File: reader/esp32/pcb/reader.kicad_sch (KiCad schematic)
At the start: 12 parts, among them U1 ESP32-WROOM-32U, U2 RDM6300

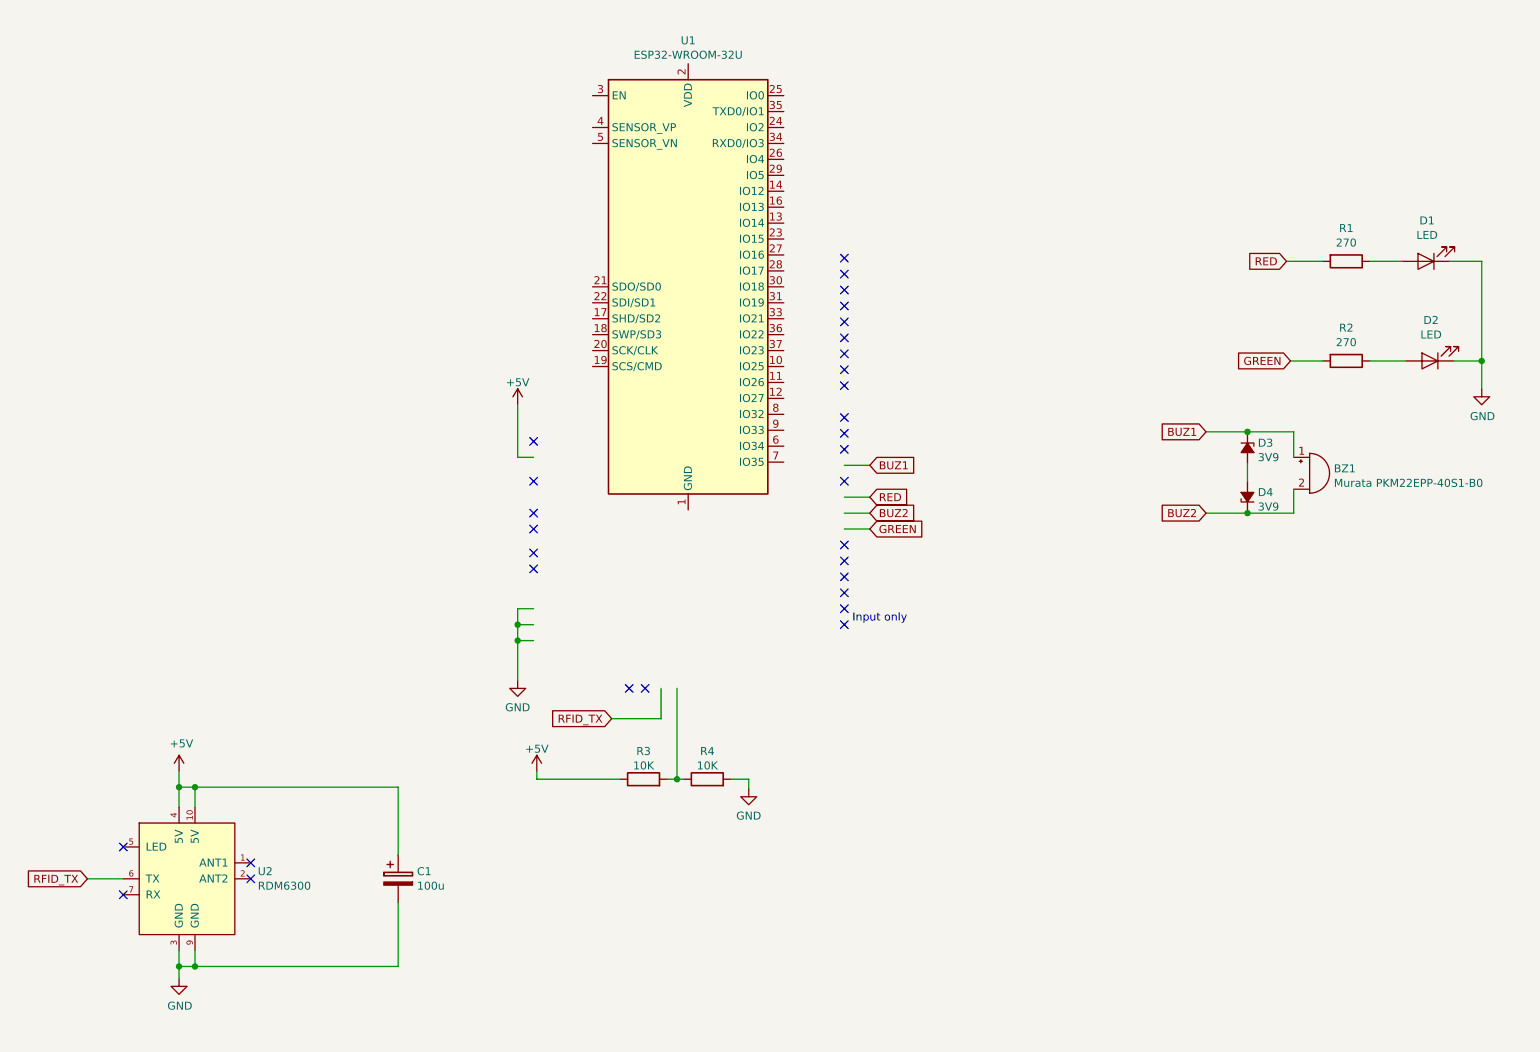
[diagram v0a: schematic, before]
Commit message: Work.
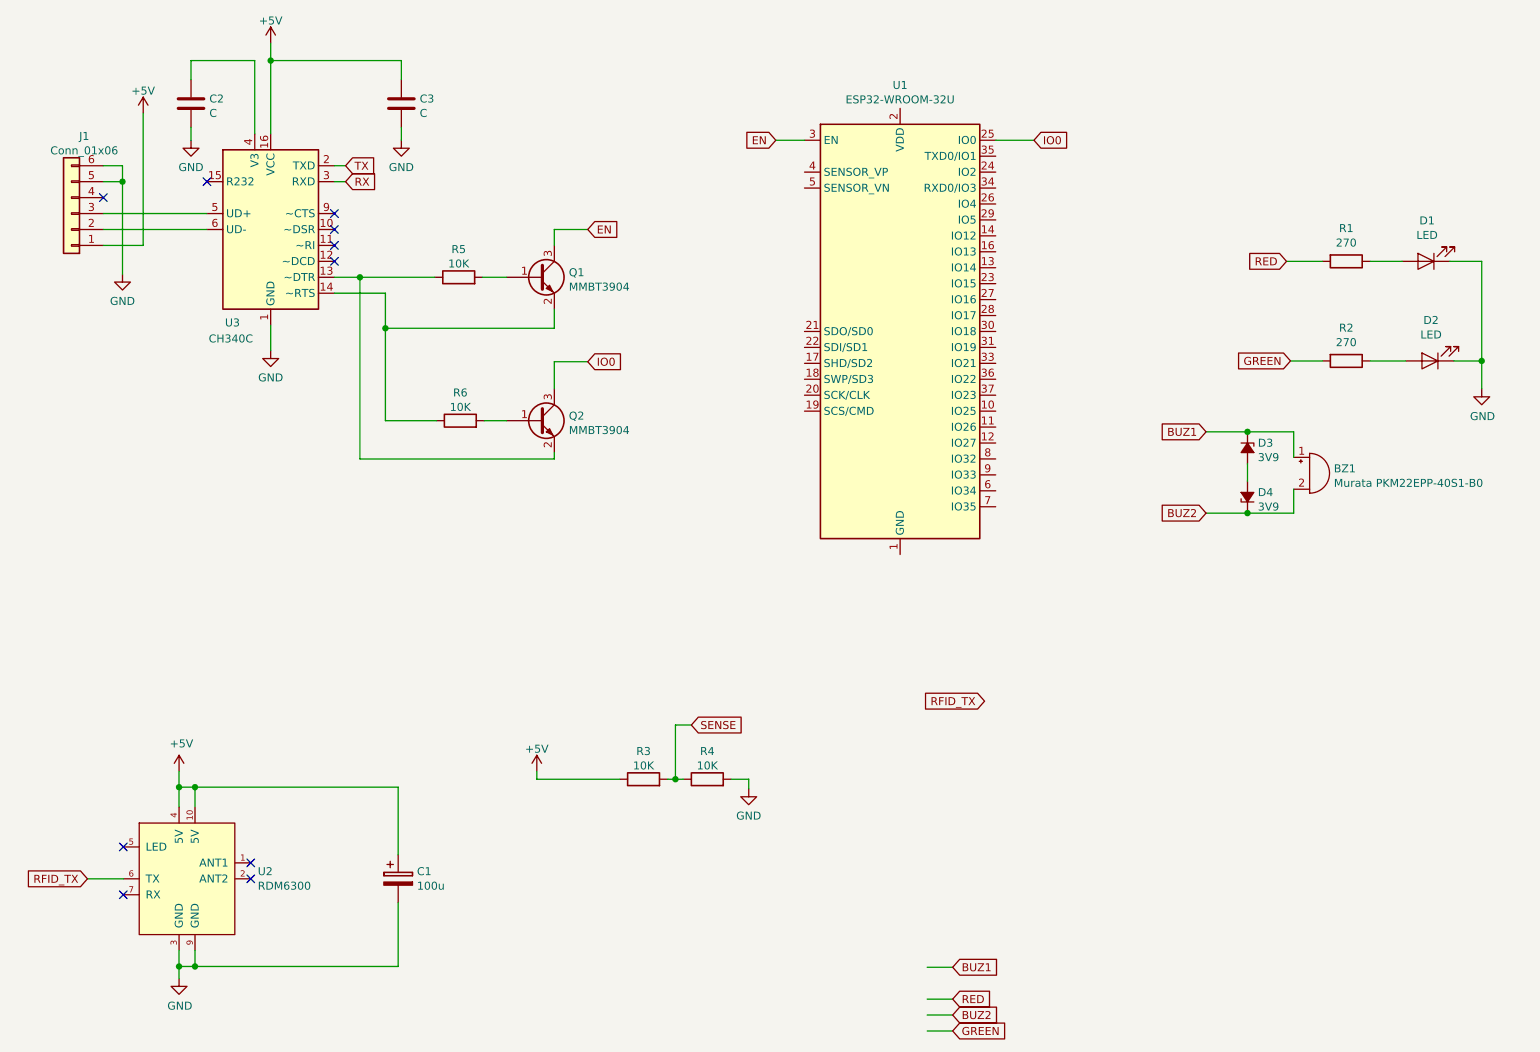
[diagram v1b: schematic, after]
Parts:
- added C2, C3: C, symbol Device:C
- added J1: Conn_01x06, Connector_USB:USB_Micro-B_Molex-105017-0001, symbol Connector_Generic:Conn_01x06
- added Q1, Q2: MMBT3904, Package_TO_SOT_SMD:SOT-23, symbol Device:Q_NPN_BEC
- added R5, R6: 10K, symbol Device:R
- added U3: CH340C, Package_SO:SOIC-16_3.9x9.9mm_P1.27mm, symbol Interface_USB:CH340C
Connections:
- net +5V: now also C3.1, J1.1 (Pin_1), U3.16 (VCC)
- net GND: now also C2.2, C3.2, J1.5 (Pin_5), J1.6 (Pin_6), U3.1 (GND)
- net IO0: now reaches U1.25 (IO0)
- net IO0: now also Q2.3 (C)
- net EN: now reaches U1.3 (EN)
- net EN: now also Q1.3 (C)
- net SENSE: now reaches R3.2, R4.1
- new net: Q1.2 (E), R6.1, U3.14 (~RTS)
- new net: Q2.1 (B), R6.2
- new net: C2.1, U3.4 (V3)
- new net: J1.2 (Pin_2), U3.6 (UD-)
- new net: J1.3 (Pin_3), U3.5 (UD+)
- new net: Q2.2 (E), R5.1, U3.13 (~DTR)
- new net: Q1.1 (B), R5.2
- new net RX: U3.3 (RXD)
- new net TX: U3.2 (TXD)
- no-connect marks 31 -> 10
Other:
- note removed: "Input only"
- moved on the sheet: U1
